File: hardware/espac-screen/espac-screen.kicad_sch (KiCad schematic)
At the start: 8 parts, among them J1 Conn_01x07, J2 GC9A01, Q1 2N7002

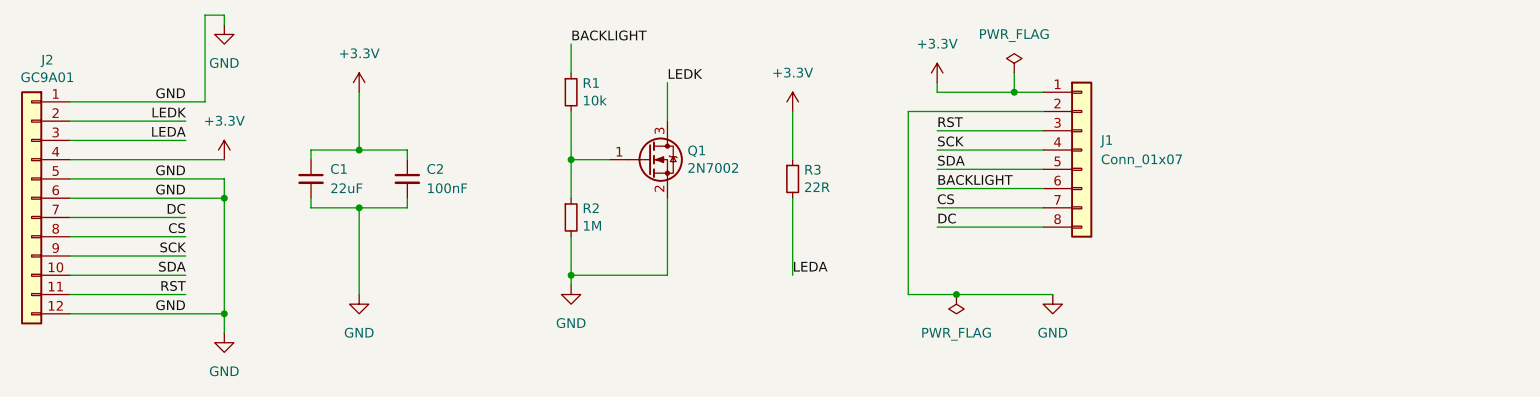
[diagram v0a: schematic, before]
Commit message: pcb updates
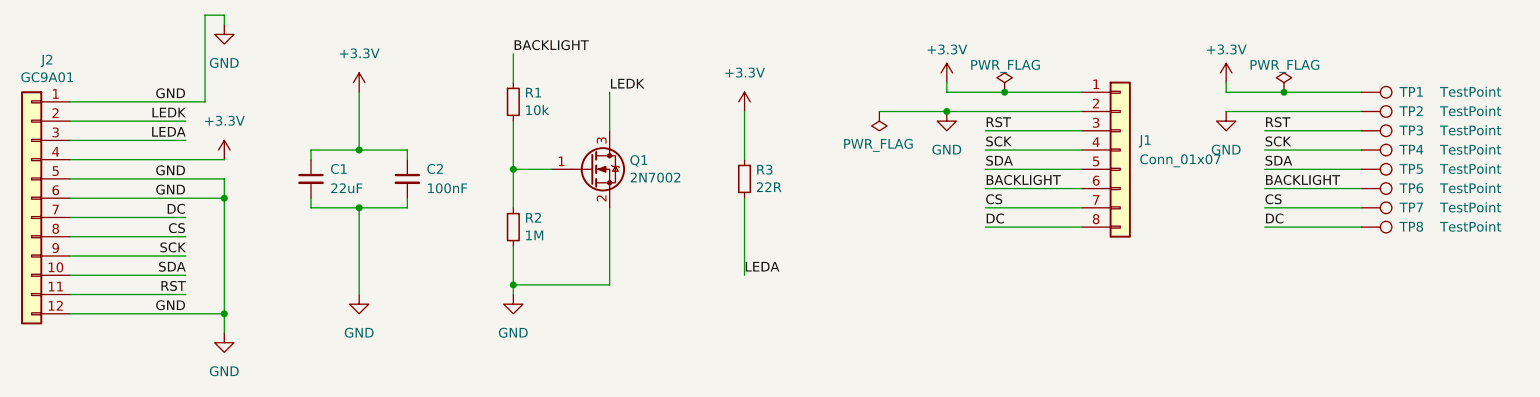
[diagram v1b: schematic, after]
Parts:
- added TP1, TP2, TP3, TP4, TP5, TP6, TP7, TP8: TestPoint, TestPoint:TestPoint_Pad_D1.5mm, symbol Connector:TestPoint
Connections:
- net +3.3V: now also TP1.1
- net BACKLIGHT: now also TP6.1
- net CS: now also TP7.1
- net DC: now also TP8.1
- net GND: now also TP2.1
- net RST: now also TP3.1
- net SCK: now also TP4.1
- net SDA: now also TP5.1
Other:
- moved on the sheet: J1, Q1, R1, R2, R3
